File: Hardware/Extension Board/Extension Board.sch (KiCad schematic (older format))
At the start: 34 parts, among them J1 CNX_LED, J10 MODE, J11 TUNING, J12 I2C, J13 I2C, J14 SPI, J15 SD, J16 TFT, J2 CNX_LED, J3 CNX_LED, J4 CNX_LED, J5 SPARE, J6 ARDUINO_DIGITAL, J7 ARDUINO_COMMS, J8 ARDUINO_ANALOG, J9 NEXT_AGAIN, U1 74HC14

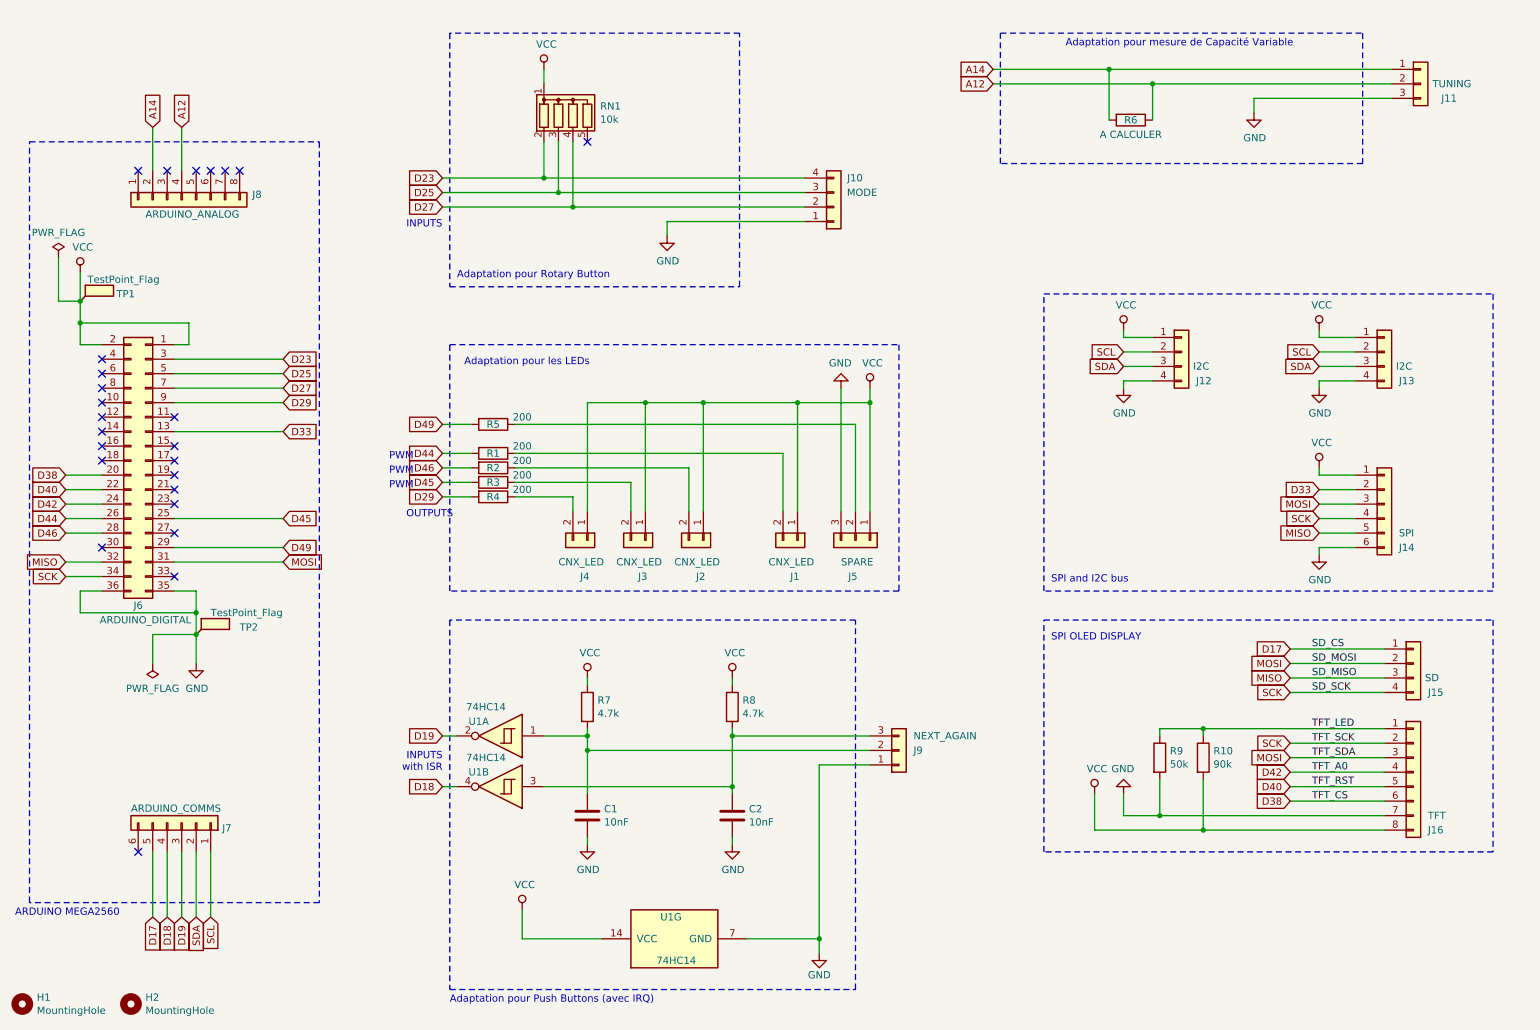
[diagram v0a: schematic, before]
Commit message: update shematics
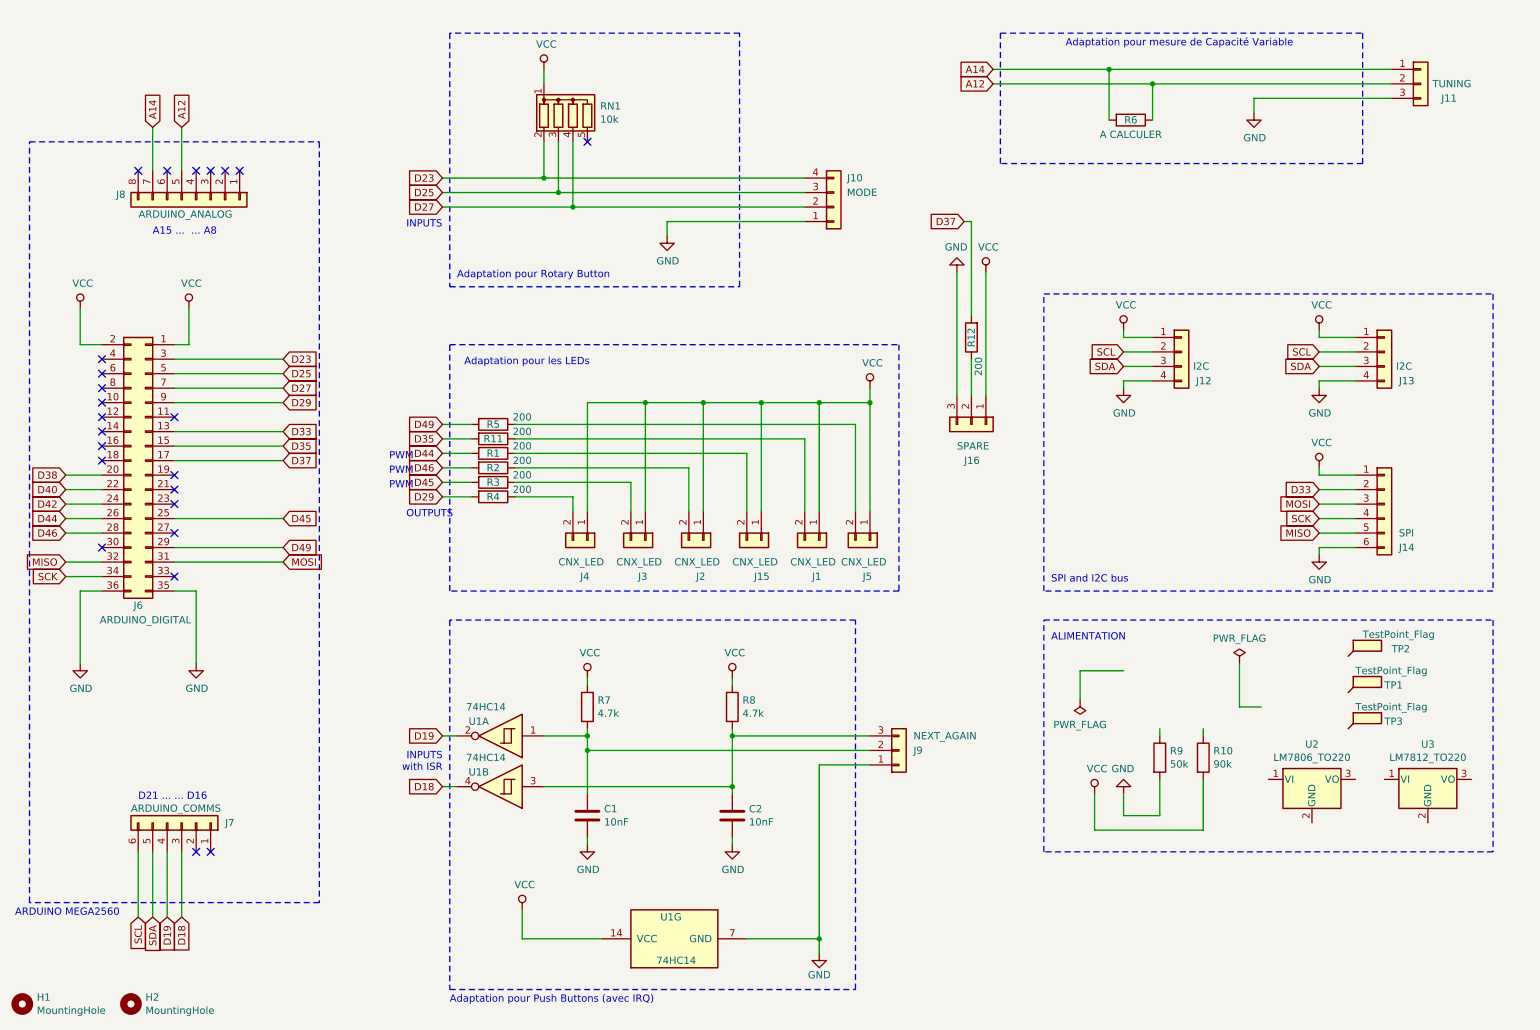
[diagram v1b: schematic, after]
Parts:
- removed J15: SD, Connector_JST:JST_XH_B4B-XH-AM_1x04_P2.50mm_Vertical, symbol Connector_Generic:Conn_01x04
- removed J16: TFT, Connector_JST:JST_XH_B8B-XH-AM_1x08_P2.50mm_Vertical, symbol Connector_Generic:Conn_01x08
- added J15, J5: CNX_LED, Connector_JST:JST_XH_B2B-XH-A_1x02_P2.50mm_Vertical, symbol Connector_Generic:Conn_01x02
- added R11, R12: 200, Resistor_THT:R_Axial_DIN0207_L6.3mm_D2.5mm_P10.16mm_Horizontal, symbol Device:R
- added TP3: TestPoint_Flag, TestPoint:TestPoint_Loop_D2.54mm_Drill1.5mm_Beaded, symbol Connector:TestPoint_Flag
- added U2: LM7806_TO220, Package_TO_SOT_THT:TO-220-3_Vertical, symbol Regulator_Linear:LM7806_TO220
- added U3: LM7812_TO220, Package_TO_SOT_THT:TO-220-3_Vertical, symbol Regulator_Linear:LM7812_TO220
- renumbered J5 to J16
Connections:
- net D17 is gone; now on net SDA: J7.5 (Pin_5)
- net A12: now also J8.5 (Pin_5); no longer J8.4 (Pin_4)
- net A14: now also J8.7 (Pin_7); no longer J8.2 (Pin_2)
- net D18: now also J7.3 (Pin_3); no longer J7.4 (Pin_4)
- net D19: now also J7.4 (Pin_4); no longer J7.3 (Pin_3)
- net GND: no longer TP2.1
- net SCL: now also J7.6 (Pin_6); no longer J7.1 (Pin_1)
- net SDA: no longer J7.2 (Pin_2)
- net VCC: now also J15.1 (Pin_1), J5.1 (Pin_1); no longer TP1.1
- net at J1.2 (Pin_2): now also R11.1; no longer R1.1
- net at J16.2 (Pin_2): now also R12.1; no longer R5.1
- net D35: now reaches J6.15 (Pin_15)
- net D35: now also R11.2
- net D37: now reaches J6.17 (Pin_17)
- net D37: now also R12.2
- net TFT_LED: no longer names the net of R9.1
- net TFT_LED: no longer R10.1
- new net: J15.2 (Pin_2), R1.1
- new net: J5.2 (Pin_2), R5.1
- no-connect marks 25 -> 24
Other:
- note added: "A15 ... ... A8"
- note added: "ALIMENTATION"
- note added: "D21 ... ... D16"
- note removed: "SPI OLED DISPLAY"
- moved on the sheet: J1, J16, TP1, TP2

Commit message: Ajout FootPrint Library MesModules
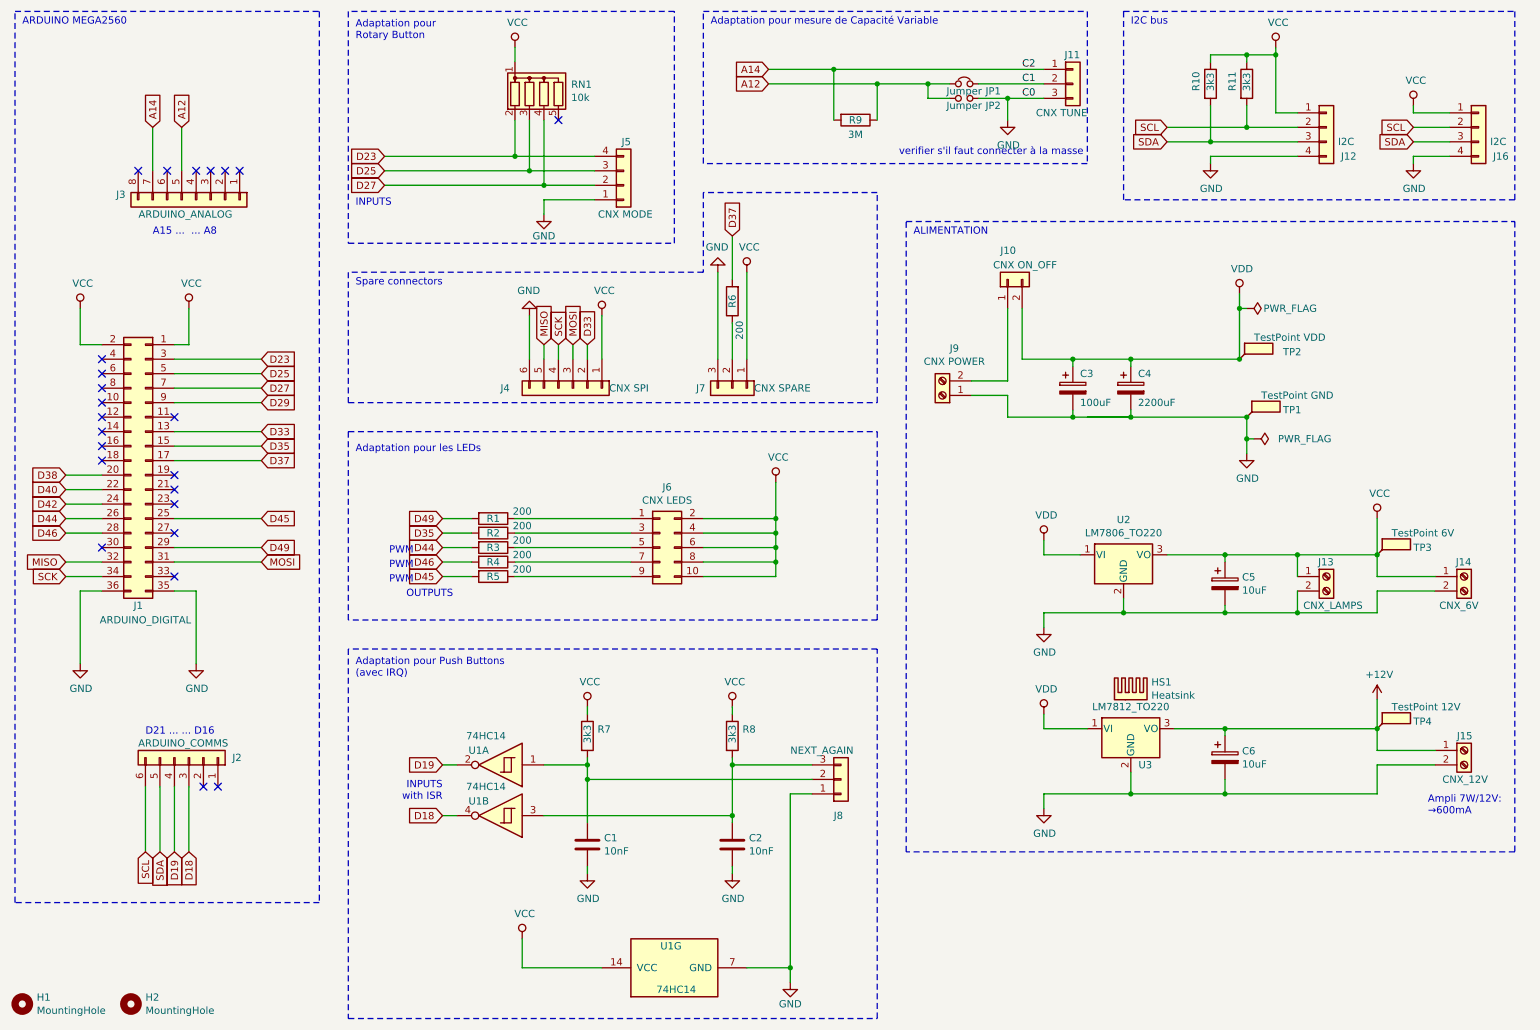
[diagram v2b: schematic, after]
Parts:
- removed J1, J15, J2, J3, J4, J5: CNX_LED, Connector_JST:JST_XH_B2B-XH-A_1x02_P2.50mm_Vertical, symbol Connector_Generic:Conn_01x02
- removed R4: 200, Resistor_THT:R_Axial_DIN0207_L6.3mm_D2.5mm_P10.16mm_Horizontal, symbol Device:R
- removed R9: 50k, Resistor_THT:R_Axial_DIN0207_L6.3mm_D2.5mm_P10.16mm_Horizontal, symbol Device:R
- added C3: 100uF, Capacitor_THT:CP_Axial_L18.0mm_D8.0mm_P25.00mm_Horizontal, symbol Device:CP
- added C4: 2200uF, Capacitor_THT:CP_Axial_L30.0mm_D18.0mm_P35.00mm_Horizontal, symbol Device:CP
- added C5, C6: 10uF, Capacitor_THT:CP_Radial_D5.0mm_P2.50mm, symbol Device:CP
- added HS1: Heatsink, MesModules:HeatSink_TO-220, symbol Mechanical:Heatsink
- added J10: CNX ON_OFF, Connector_JST:JST_XH_B2B-XH-A_1x02_P2.50mm_Vertical, symbol Connector_Generic:Conn_01x02
- added J13: CNX_LAMPS, MesModules:Bloc_de_jonction_CI-MPT_2.54mm_01x02, symbol Connector:Screw_Terminal_01x02
- added J14: CNX_6V, TerminalBlock_Phoenix:TerminalBlock_Phoenix_MKDS-1,5-2-5.08_1x02_P5.08mm_Horizontal, symbol Connector:Screw_Terminal_01x02
- added J15: CNX_12V, TerminalBlock_Phoenix:TerminalBlock_Phoenix_MKDS-1,5-2-5.08_1x02_P5.08mm_Horizontal, symbol Connector:Screw_Terminal_01x02
- added J6: CNX LEDS, symbol Connector_Generic:Conn_02x05_Odd_Even
- added J9: CNX POWER, TerminalBlock_Phoenix:TerminalBlock_Phoenix_MKDS-1,5-2-5.08_1x02_P5.08mm_Horizontal, symbol Connector:Screw_Terminal_01x02
- added JP1: Jumper, Connector_PinHeader_2.54mm:PinHeader_1x02_P2.54mm_Vertical, symbol Device:Jumper_NC_Small
- added JP2: Jumper, Connector_PinHeader_2.54mm:PinHeader_1x02_P2.54mm_Vertical, symbol Device:Jumper_NO_Small
- added R11: 3k3, Resistor_THT:R_Axial_DIN0207_L6.3mm_D2.5mm_P10.16mm_Horizontal, symbol Device:R
- added TP4: TestPoint 12V, TestPoint:TestPoint_Loop_D2.54mm_Drill1.5mm_Beaded, symbol Connector:TestPoint_Flag
- J11: value TUNING -> CNX TUNE
- J4: renamed from J14; value SPI -> CNX SPI
- J5: renamed from J10; value MODE -> CNX MODE
- J7: renamed from J16; value SPARE -> CNX SPARE; footprint Connector_JST:JST_XH_B3B-XH-A_1x03_P2.50mm_Vertical -> Connector_JST:JST_XH_B3B-XH-AM_1x03_P2.50mm_Vertical
- R10: value 90k -> 3k3
- R7, R8: value 4.7k -> 3k3
- R9: renamed from R6; value A CALCULER -> 3M; footprint Resistor_THT:R_Axial_DIN0411_L9.9mm_D3.6mm_P20.32mm_Horizontal -> (none)
- TP1: value TestPoint_Flag -> TestPoint GND
- TP2: value TestPoint_Flag -> TestPoint VDD
- TP3: value TestPoint_Flag -> TestPoint 6V
- renumbered J6 to J1, J13 to J16, J7 to J2, J8 to J3, J9 to J8, R5 to R1, R11 to R2, R1 to R3, R2 to R4, R3 to R5, R12 to R6
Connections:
- net A12: now also JP1.1, JP2.1; no longer J11.2 (Pin_2)
- net GND: now also TP1.1, U2.2 (GND), U3.2 (GND), C3.2, C4.2, C5.2, C6.2, J13.2 (Pin_2), J14.2 (Pin_2), J15.2 (Pin_2), J9.1 (Pin_1), JP2.2
- net SCL: now also R11.2
- net SDA: now also R10.2
- net VCC: now also R10.1, TP3.1, U2.3 (VO), C5.1, J13.1 (Pin_1), J14.1 (Pin_1), J6.10 (Pin_10), J6.2 (Pin_2), J6.4 (Pin_4), J6.6 (Pin_6), J6.8 (Pin_8), R11.1; no longer R10.2
- net at R5.1: now also J6.9 (Pin_9)
- net at R4.1: now also J6.7 (Pin_7)
- net at R2.1: now also J6.3 (Pin_3)
- net VDD: now reaches TP2.1
- net VDD: now also U2.1 (VI), U3.1 (VI), C3.1, C4.1, J10.2 (Pin_2)
- net at R3.1: now also J6.5 (Pin_5)
- net at R1.1: now also J6.1 (Pin_1)
- net +12V: now reaches U3.3 (VO)
- net +12V: now also C6.1, J15.1 (Pin_1), TP4.1
- new net: J10.1 (Pin_1), J9.2 (Pin_2)
- new net C1: J11.2 (Pin_2), JP1.2
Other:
- note added: "Adaptation pour Push Buttons \n(avec IRQ)"
- note added: "Adaptation pour \nRotary Button"
- note added: "Ampli 7W/12V:\n→600mA"
- note added: "I2C bus"
- note added: "Spare connectors"
- note added: "verifier s'il faut connecter à la masse"
- note removed: "Adaptation pour Push Buttons (avec IRQ)"
- note removed: "Adaptation pour Rotary Button"
- note removed: "SPI and I2C bus"
- moved on the sheet: C1, C2, J11, J12, J16, J2, J4, J5, J7, J8, R1, R2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
